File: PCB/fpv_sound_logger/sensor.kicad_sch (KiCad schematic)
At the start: 10 parts, among them U2 INMP441ACEZ-R7

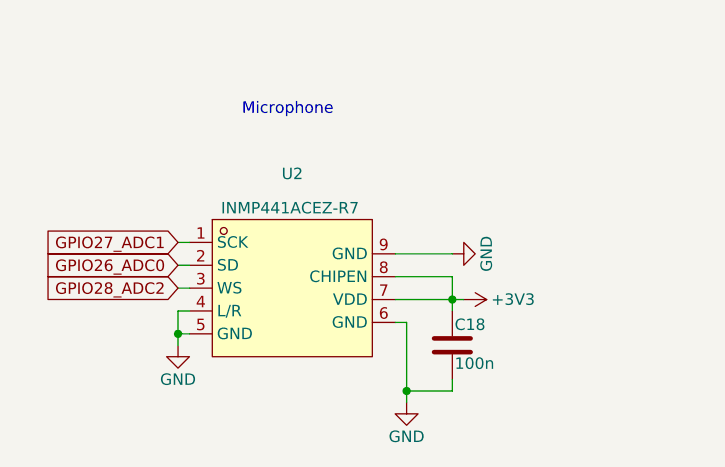
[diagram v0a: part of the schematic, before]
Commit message: Refactor code structure for improved readability and maintainability
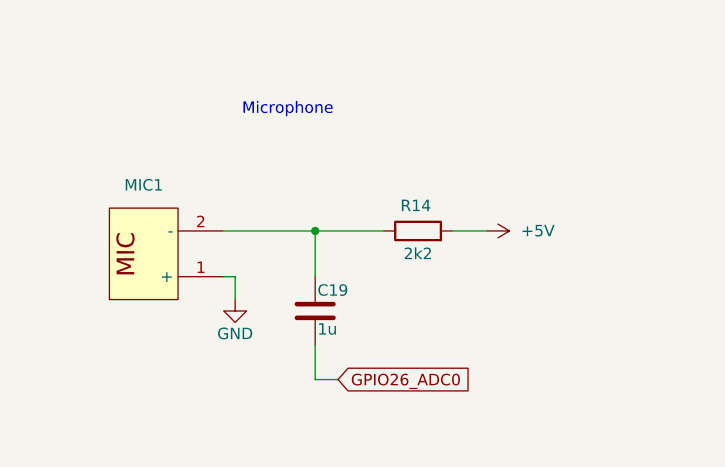
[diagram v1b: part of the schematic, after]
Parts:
- removed C18: 100n, Capacitor_SMD:C_0603_1608Metric, symbol Device:C
- removed U2: INMP441ACEZ-R7, fpv_sound_logger:MID-SMD_L4.7-W3.8_INMP441ACEZ, symbol SoundLogger:INMP441ACEZ-R7
- added C19: 1u, Capacitor_SMD:C_0603_1608Metric, symbol Device:C
- added MIC1: (no value), fpv_sound_logger:MIC-TH_BD6.0-P1.90-D0.4-L-FD_GMI6050P-2CXXDB, symbol SoundLogger:GMI6050P-36DB
- added R14: 2k2, Resistor_SMD:R_0603_1608Metric, symbol Device:R
- LED1: MANUFACTURER (none) -> EVERLIGHT; Manufacturer_Part_Number IN-S66TFT5R5G5B -> 19-337/R6GHBHC-A01/2T; Supplier (none) -> LCSC; Supplier Part (none) -> C264519
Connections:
- net +5V: now also R14.2
- net GND: now also MIC1.1 (+)
- net GPIO26_ADC0: now also C19.2
- new net: C19.1, MIC1.2 (-), R14.1
